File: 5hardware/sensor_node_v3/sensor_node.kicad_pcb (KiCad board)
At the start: 2 copper layers, 50.9 x 100.1 mm, 30 parts, among them J1 Conn_01x03, J3 Conn_01x29, SW1 SW_Push, SW2 SW_DIP_x04, SW4 SW_DIP_x04, SW5 RotaryEncoder, SW6 SW_Push, U1 MCP1700x-330xxTO, U7 CH32V003F4P6, U8 ESP32-WROOM-32D

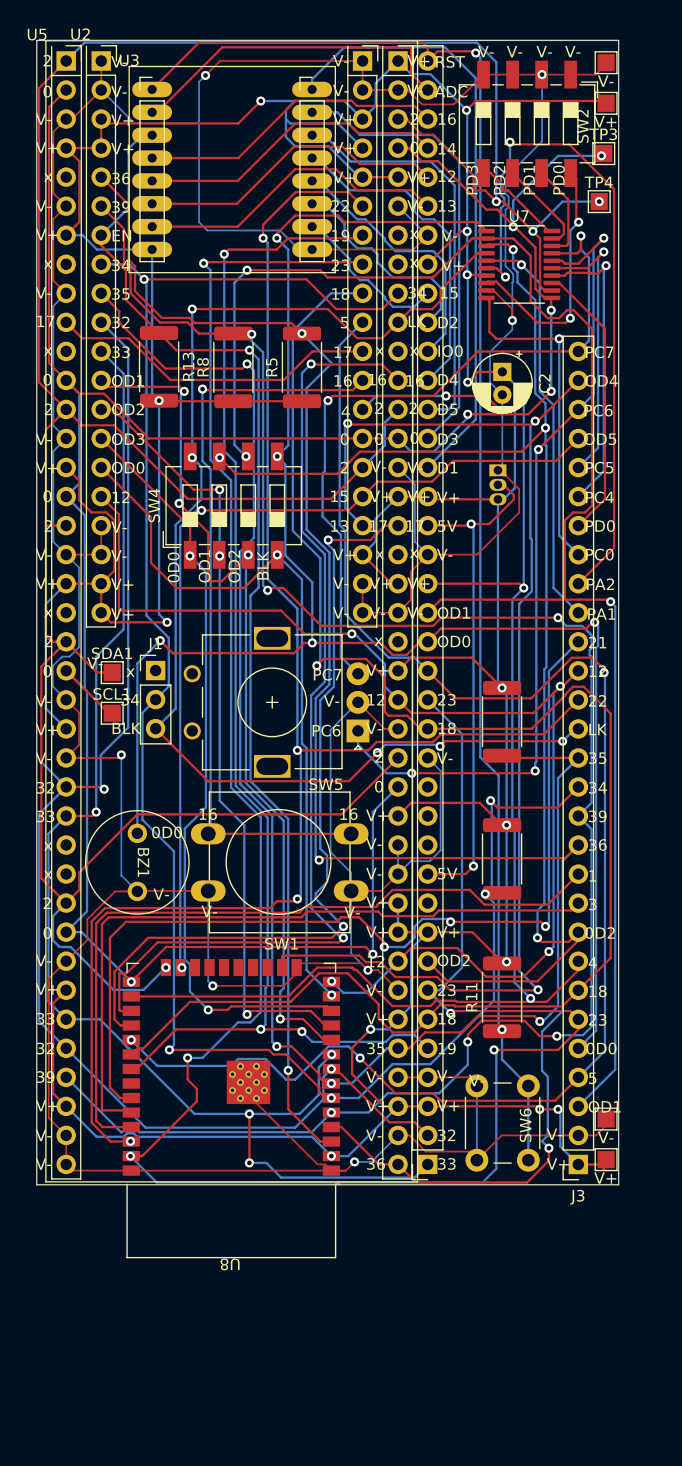
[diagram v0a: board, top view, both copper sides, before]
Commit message: fixing pcb design.
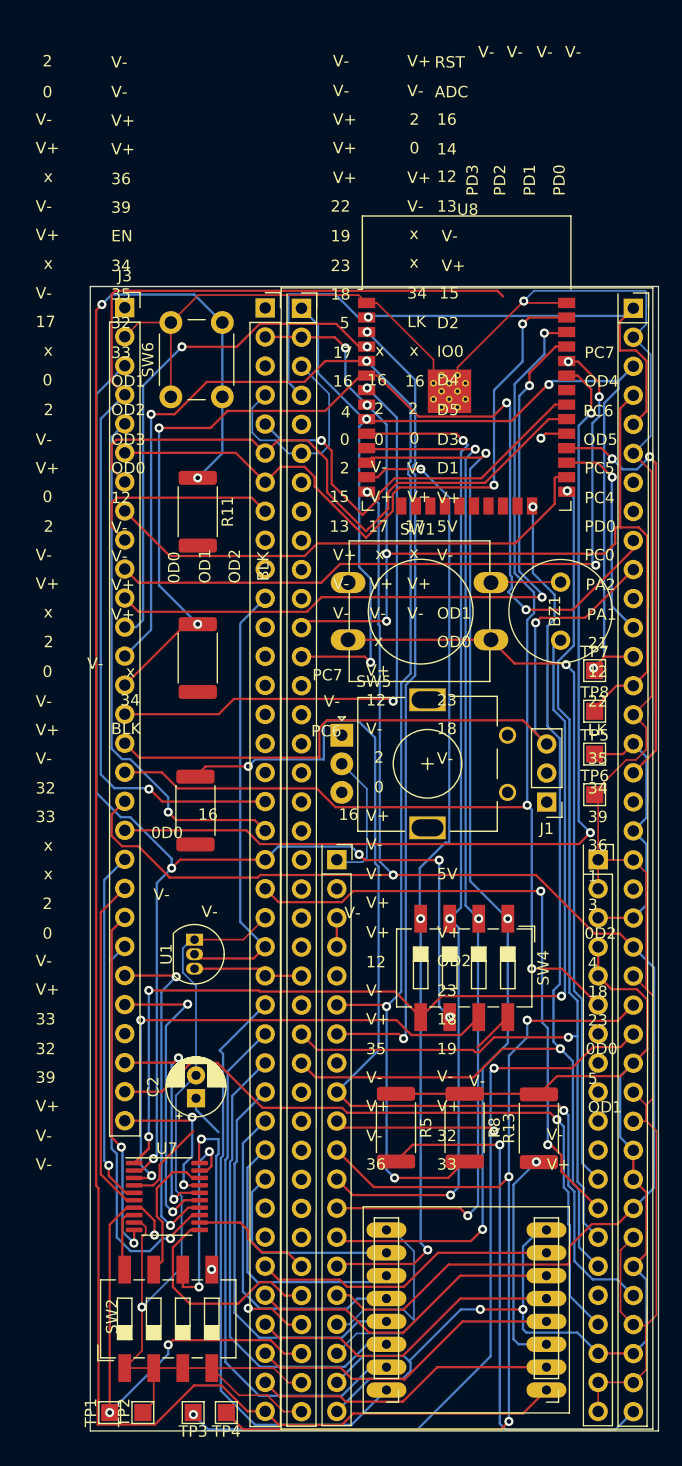
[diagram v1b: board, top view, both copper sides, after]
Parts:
- removed SCL1, SDA1, V+ (x2), V- (x2): TestPoint, TestPoint:TestPoint_Pad_1.5x1.5mm
- added TP1: TestPoint, TestPoint:TestPoint_Pad_1.5x1.5mm, F.Cu at (92.2, 152.9)
- added TP2: TestPoint, TestPoint:TestPoint_Pad_1.5x1.5mm, F.Cu at (95.1, 152.9)
- added TP5: TestPoint, TestPoint:TestPoint_Pad_1.5x1.5mm, F.Cu at (134.6, 95.3)
- added TP6: TestPoint, TestPoint:TestPoint_Pad_1.5x1.5mm, F.Cu at (134.6, 98.9)
- added TP7: TestPoint, TestPoint:TestPoint_Pad_1.5x1.5mm, F.Cu at (134.6, 88.0)
- added TP8: TestPoint, TestPoint:TestPoint_Pad_1.5x1.5mm, F.Cu at (134.6, 91.6)
- U1: moved to F.Cu
- moved U3 123.9 mm to (132.4, 153.0), turned to 180 degrees
- moved TP3 115.8 mm to (99.5, 152.9), turned to 180 degrees
- moved TP4 110.8 mm to (102.4, 152.9), turned to 180 degrees
- moved SW2 109.1 mm to (97.3, 144.7), turned to 90 degrees
- moved U8 93.6 mm to (123.5, 48.2), turned to 0 degrees
- moved U7 87.2 mm to (97.2, 134.0)
- moved J3 84.8 mm to (93.5, 56.3), turned to 0 degrees
- moved U4 76.3 mm to (105.8, 56.3), turned to 0 degrees
- moved R13 74.4 mm to (129.7, 128.1), turned to 90 degrees
- moved U2 72.8 mm to (110.2, 102.8)
- moved SW6 71.9 mm to (97.5, 64.1)
- moved R8 69.5 mm to (123.2, 128.0), turned to -90 degrees
- moved C2 69.0 mm to (99.7, 125.4), turned to 90 degrees
- moved R5 67.0 mm to (117.2, 128.0), turned to -90 degrees
- moved R11 50.1 mm to (99.9, 74.1), turned to -90 degrees
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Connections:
- TP3 pad 1: SCL1 (0) -> SCL (32)
- TP4 pad 1: SDA1 (2) -> SDA (33)
- U5 pad 1: SDA1 (2) -> SDA (33)
- U5 pad 12: SCL1 (0) -> SCL (32)
- U5 pad 13: SDA1 (2) -> SDA (33)
- U5 pad 16: SCL1 (0) -> SCL (32)
- U5 pad 17: SDA1 (2) -> SDA (33)
- U5 pad 2: SCL1 (0) -> SCL (32)
- U5 pad 21: SDA1 (2) -> SDA (33)
- U5 pad 22: SCL1 (0) -> SCL (32)
- U5 pad 26: SCL (32) -> SCL1 (0)
- U5 pad 27: SDA (33) -> SDA1 (2)
- U5 pad 30: SDA1 (2) -> SDA (33)
- U5 pad 31: SCL1 (0) -> SCL (32)
- U5 pad 34: SDA (33) -> SDA1 (2)
- U5 pad 35: SCL (32) -> SCL1 (0)
- U5 pad 42: SDA1 (2) -> SDA (33)
- U5 pad 43: SCL1 (0) -> SCL (32)
- U5 pad 52: SDA1 (2) -> SDA (33)
- U5 pad 53: SCL1 (0) -> SCL (32)
- U5 pad 64: SDA1 (2) -> SDA (33)
- U5 pad 65: SCL1 (0) -> SCL (32)
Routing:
- net +3.3V: track 409.8 -> 249.5 mm, vias 14 -> 6
- net SDA1 (2): track 255.6 -> 105.2 mm, vias 4 -> 2
- net MOSI (23): track 197.8 -> 59.0 mm, vias 5 -> 2
- net GND: track 467.7 -> 340.8 mm, vias 7 -> 2
- net SCL1 (0): track 219.6 -> 112.6 mm, vias 7 -> 2
- net SCK (18): track 142.6 -> 54.6 mm, vias 1 -> 0
- net OD5 (15): track 76.8 -> 0.00 mm, vias 2 -> 0
- net MISO (19): track 111.0 -> 35.6 mm, vias 3 -> 1
- net SDA (33): track 115.2 -> 184.8 mm, vias 4 -> 7
- net TX2 (16): track 86.5 -> 18.5 mm, vias 2 -> 1
- net IO_34: track 159.5 -> 92.8 mm, vias 5 -> 4
- net SCL (32): track 114.4 -> 178.1 mm, vias 2 -> 7
- net IO_36: track 151.5 -> 91.6 mm
- net Net-(J3-Pin_27): track 73.1 -> 20.1 mm, vias 4 -> 2
- net OD2: track 115.4 -> 64.5 mm, vias 4 -> 2
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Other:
- board size 50.9 x 100.1 mm -> 49.7 x 100.1 mm
